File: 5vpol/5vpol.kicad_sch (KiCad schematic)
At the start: 31 parts, among them J1 IN, J2 OUT, U1 TPS62135

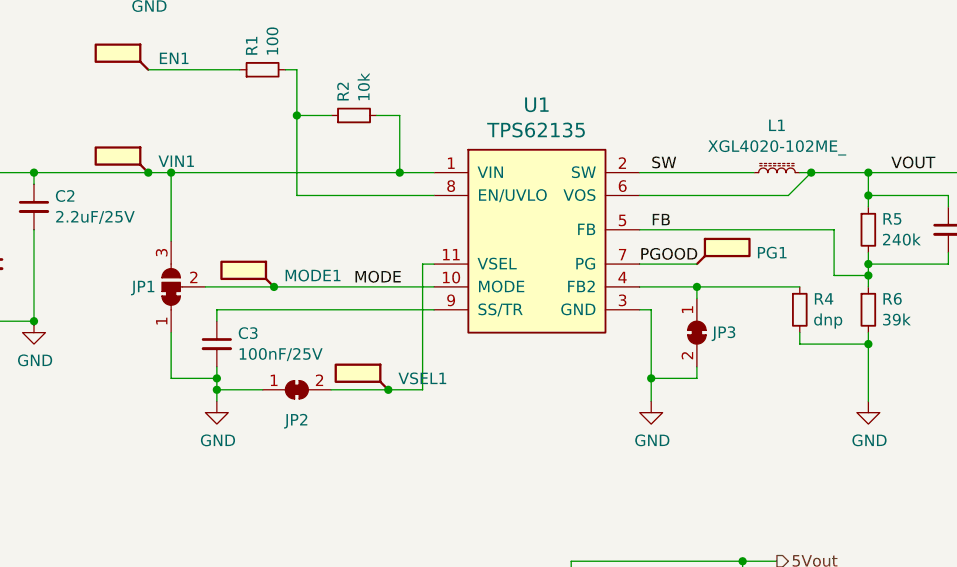
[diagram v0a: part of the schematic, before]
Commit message: Reapply "Update modules to kicad v7 format"
This reverts commit fa5cc85431189ac7a3beedf0871b5723203ae43f.
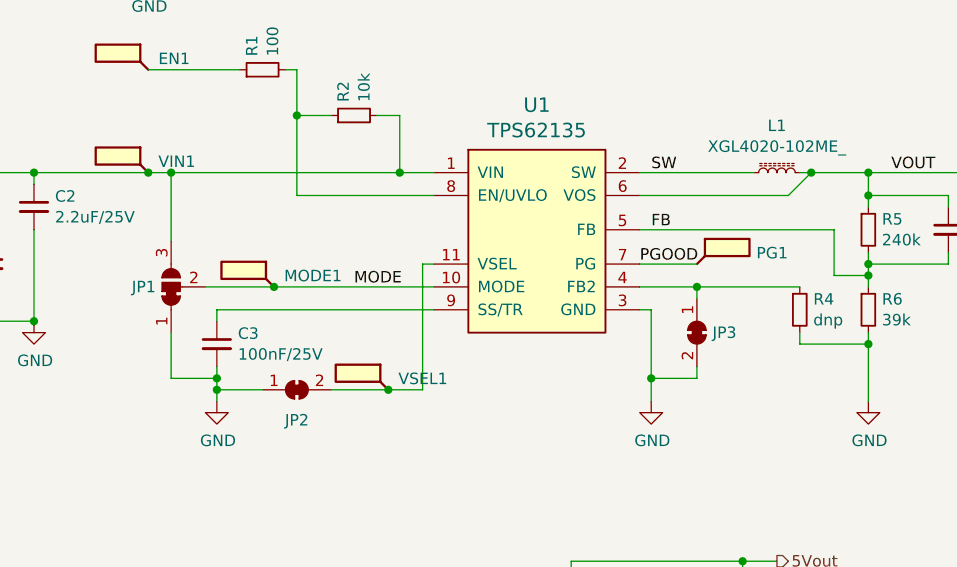
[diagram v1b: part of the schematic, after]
